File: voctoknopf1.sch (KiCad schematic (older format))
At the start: 12 parts

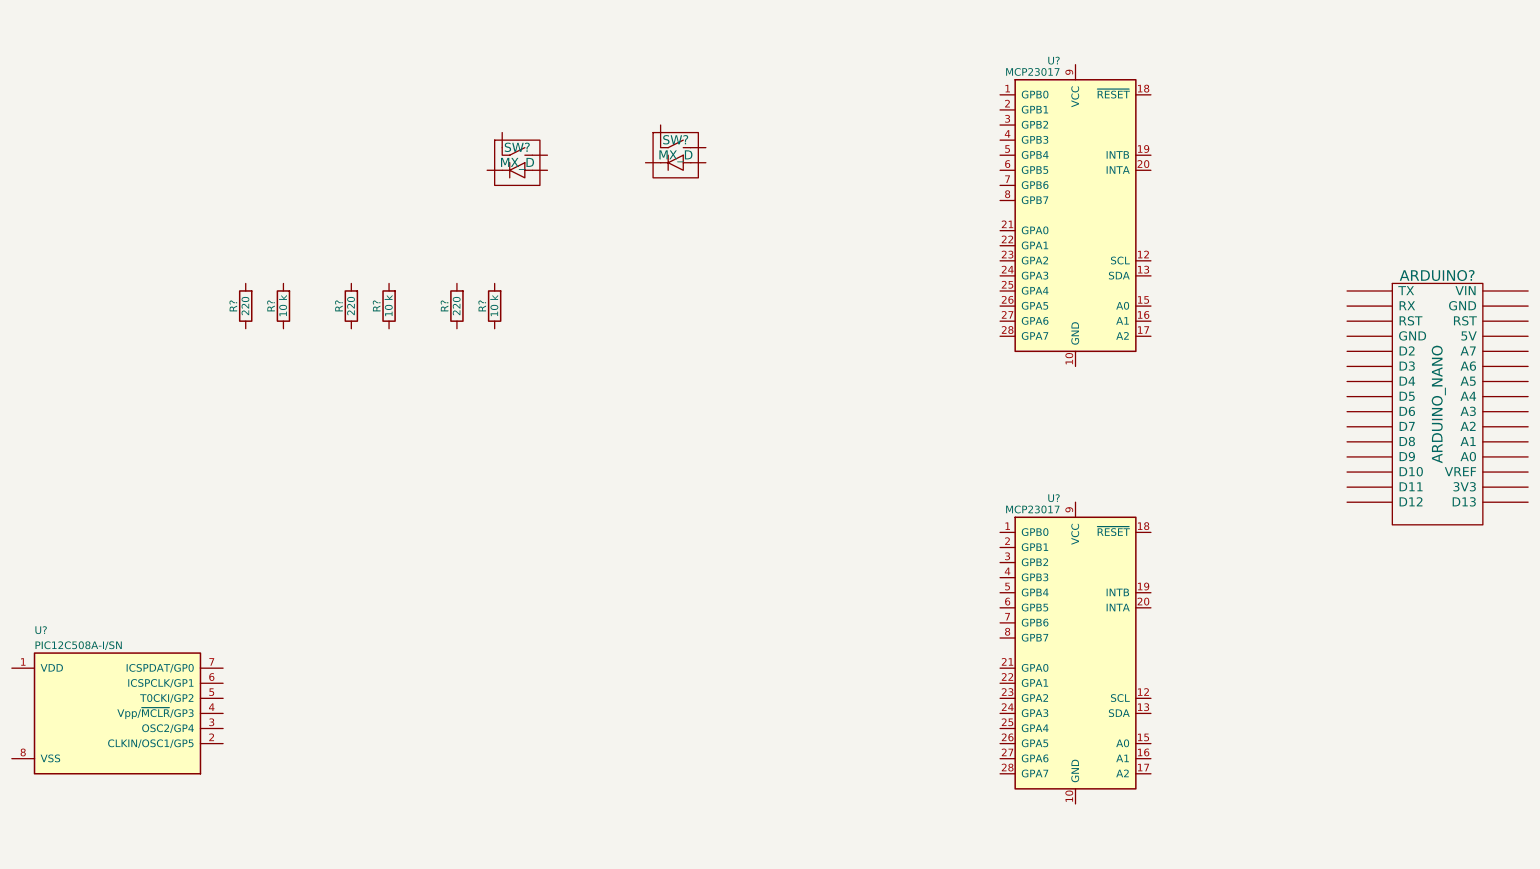
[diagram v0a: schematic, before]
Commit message: pcb weiter machen
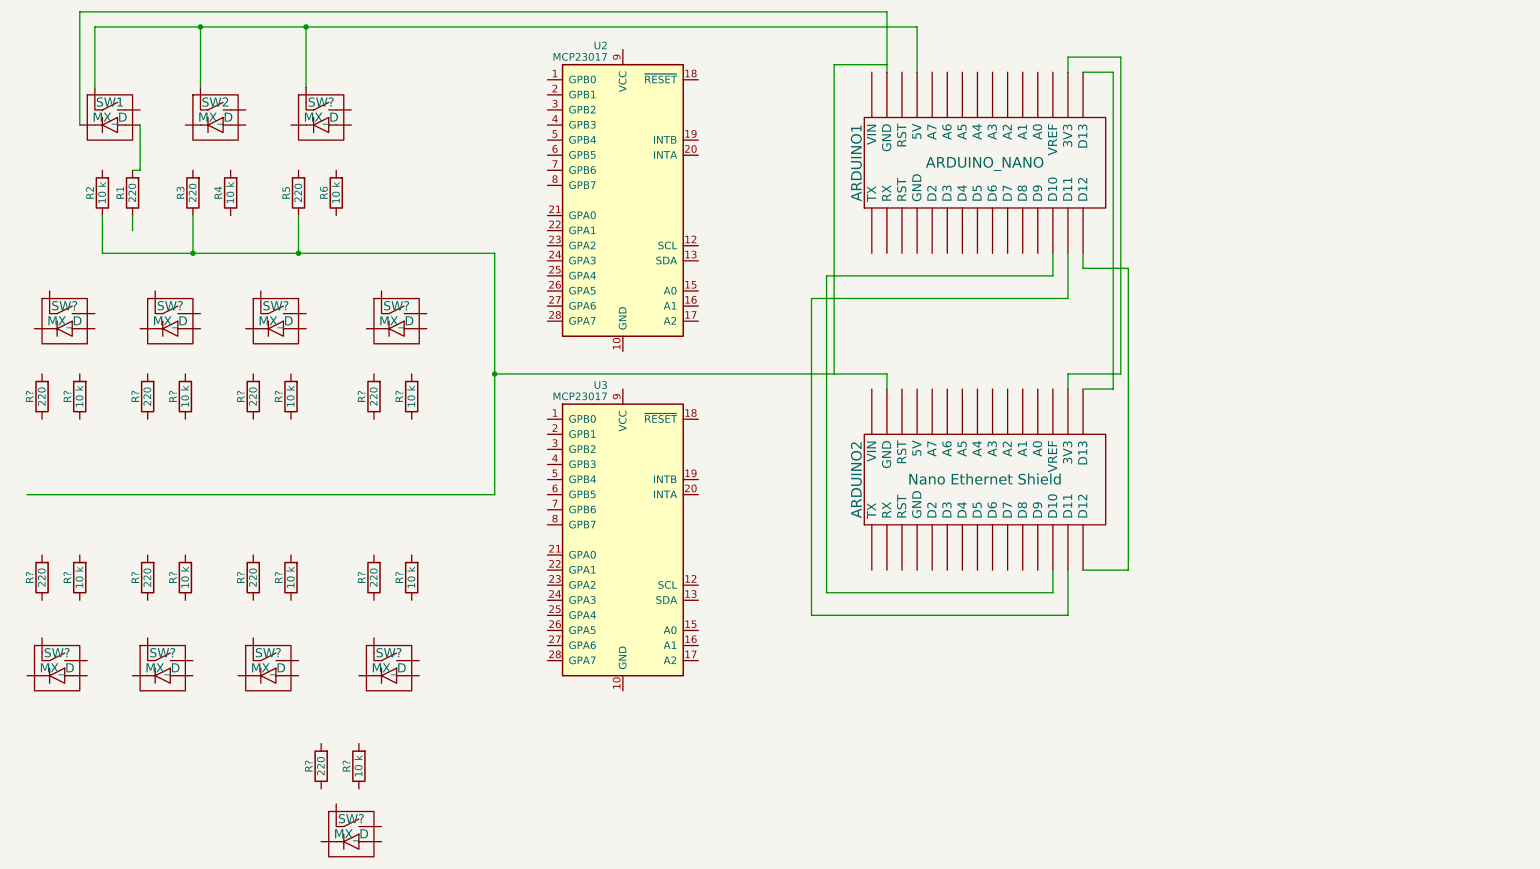
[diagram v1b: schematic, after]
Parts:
- removed U?: PIC12C508A-I/SN, symbol PIC12C508A-I/SN
- added ARDUINO1: ARDUINO_NANO, symbol ARDUINO_NANO
- added R? (x9): 10 k, symbol R
- added R? (x9): 220, symbol R
- added SW? (x10): MX_D, symbol MX_D
- ARDUINO2: renamed from ARDUINO?; value ARDUINO_NANO -> Nano Ethernet Shield
- gave numbers to parts that had none: 10
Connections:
- wire segments 0 -> 43
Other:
- moved on the sheet: ARDUINO2, R1, R2, R3, R4, R5, R6, SW1, SW2, U2, U3

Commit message: more pcb foo
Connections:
- net labels added: 5V, GND
- wire segments 43 -> 185
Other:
- moved on the sheet: R1, R2, R3, R4, R5, R6, R?, SW1, SW2, SW?, U2, U3
